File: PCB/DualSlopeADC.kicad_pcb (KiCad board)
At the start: 2 copper layers, 47 x 71.9 mm, 37 parts, among them J2 Conn_01x02_Pin, J3 Conn_01x02_Pin, J5 Conn_01x02_Pin, J6 Conn_01x02_Pin, J7 Conn_01x02_Pin, J8 Conn_01x02_Pin, J9 Conn_01x02_Pin, U1 CH32V003FxPx, U2 ADR4533, U3 AD8605ARTZ-R2, U4 ADG419BRM, U5 LTC6752xSC6-4, U6 CA56-12EWA, U7 AD8656

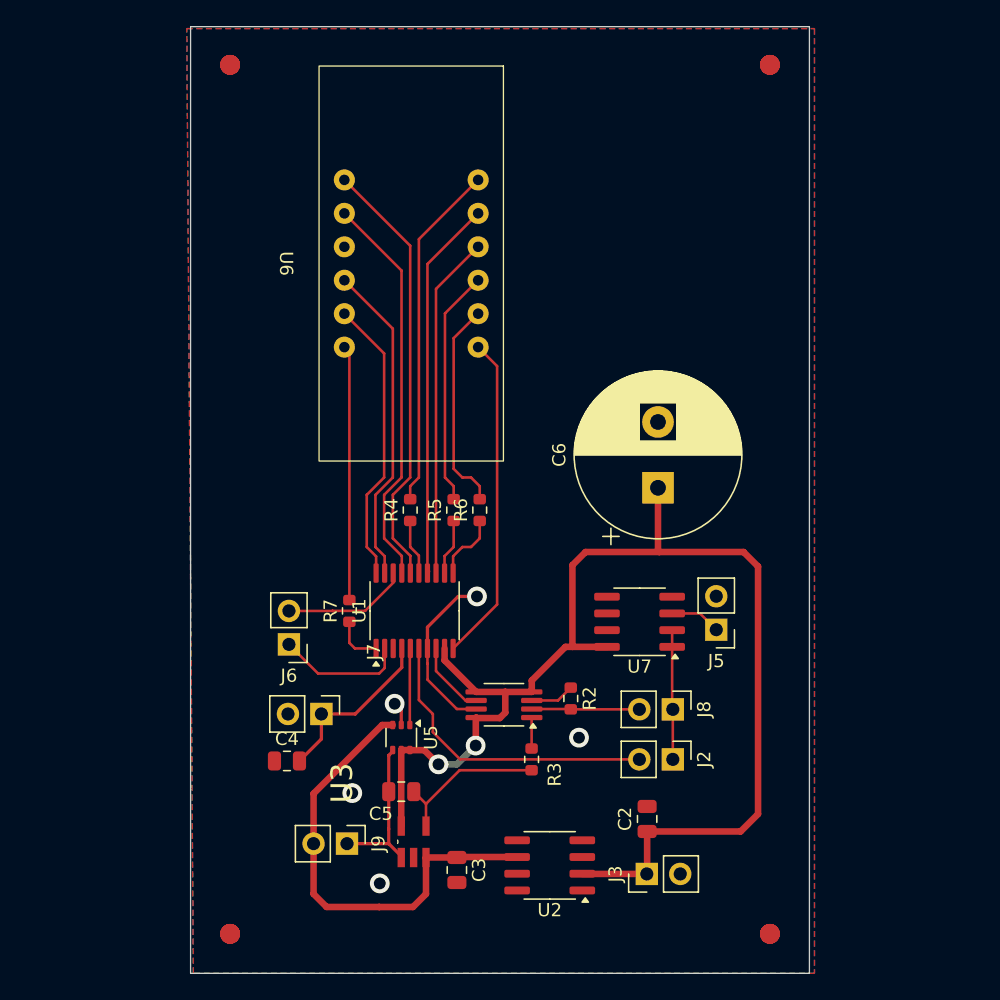
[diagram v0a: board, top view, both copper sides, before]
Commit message: visulle sachen
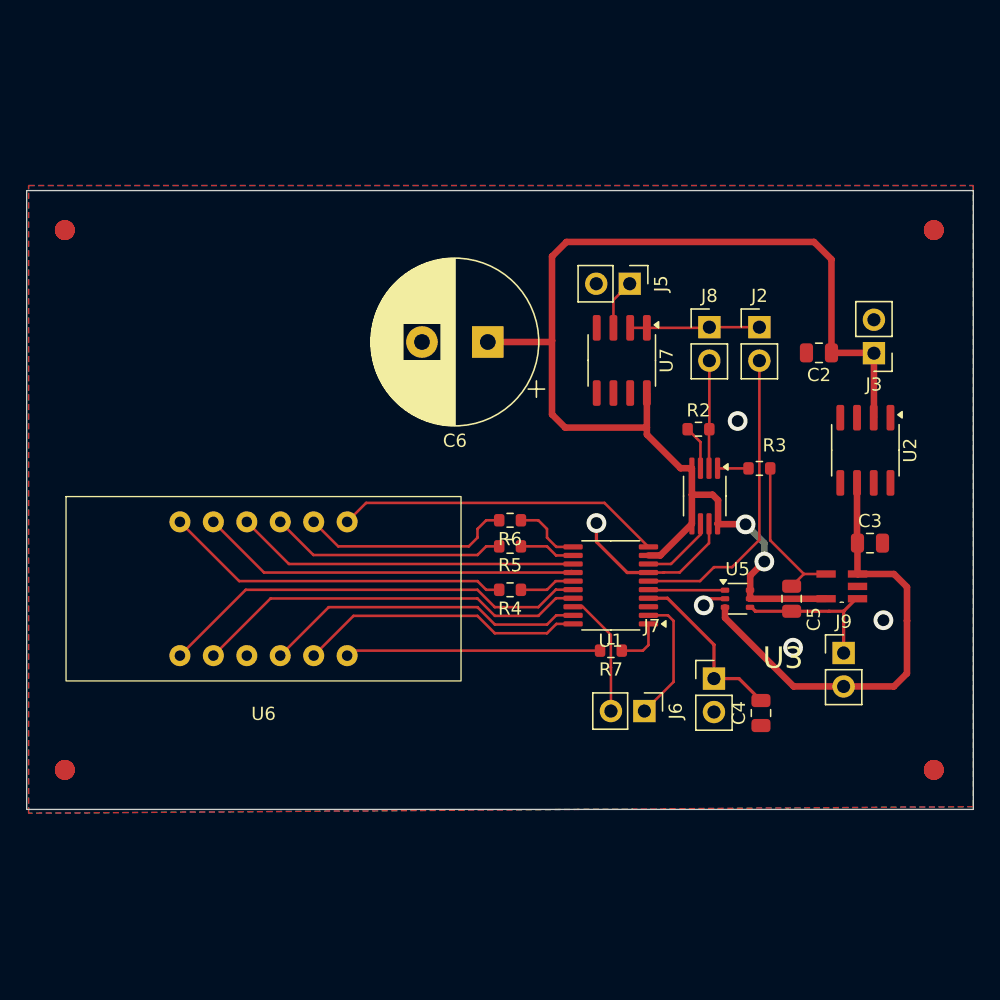
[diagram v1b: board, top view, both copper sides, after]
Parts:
- moved ? 55.0 mm to (107.8, 73.3), turned to 90 degrees (x3)
- moved ? 55.0 mm to (107.8, 114.3), turned to 90 degrees (x3)
- moved ? 54.9 mm to (173.8, 114.3), turned to 90 degrees (x3)
- moved ? 54.9 mm to (173.8, 73.3), turned to 90 degrees (x3)
- moved J3 43.1 mm to (169.2, 82.7), turned to 180 degrees
- moved J9 40.4 mm to (166.9, 105.5), turned to 0 degrees
- moved C3 40.0 mm to (168.9, 97.1), turned to 0 degrees
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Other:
- board size 47 x 71.9 mm -> 71.9 x 47 mm
